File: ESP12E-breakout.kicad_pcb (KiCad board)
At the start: 2 copper layers, 26.7 x 35.1 mm, 17 parts, among them P1 CONN_01X10, P3 CONN_01X08, SW1 RESET, SW2 FLASH, U1 ESP-12E, U2 AP1117

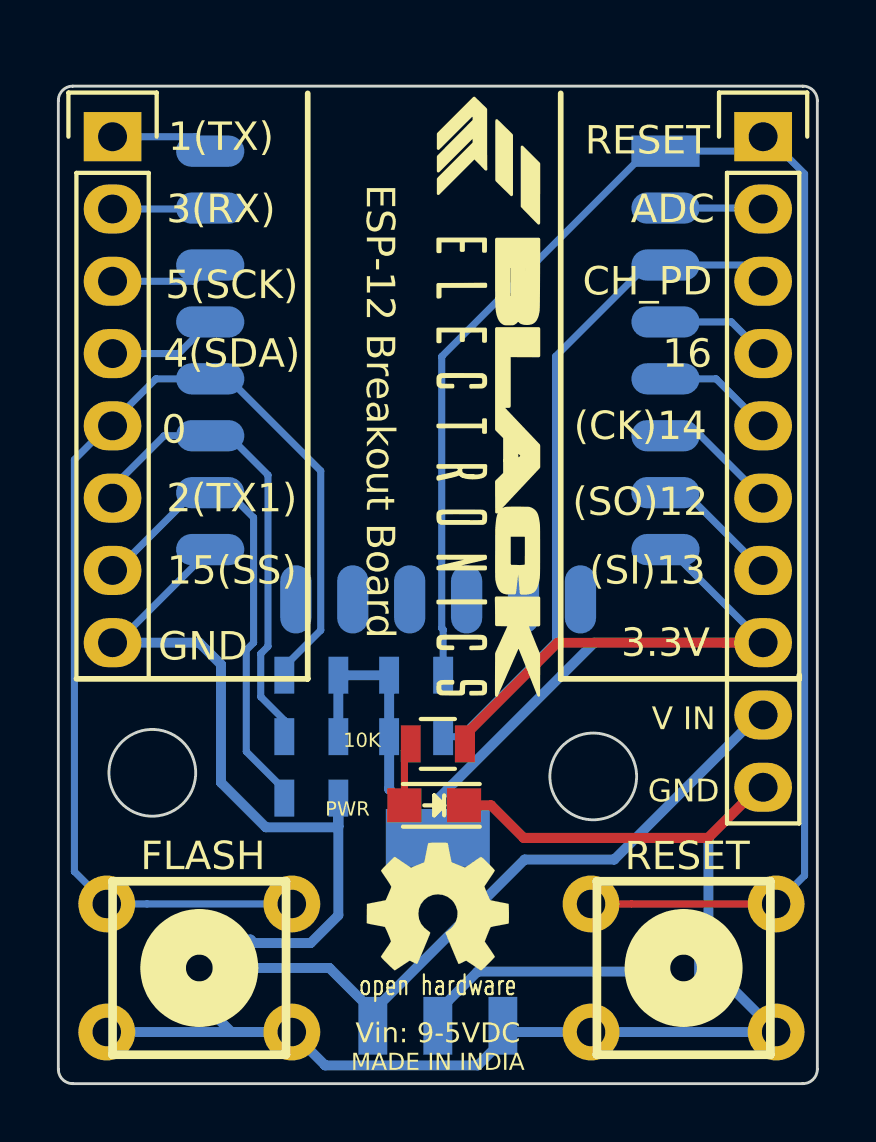
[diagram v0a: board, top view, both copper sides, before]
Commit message: Ready for prototype run
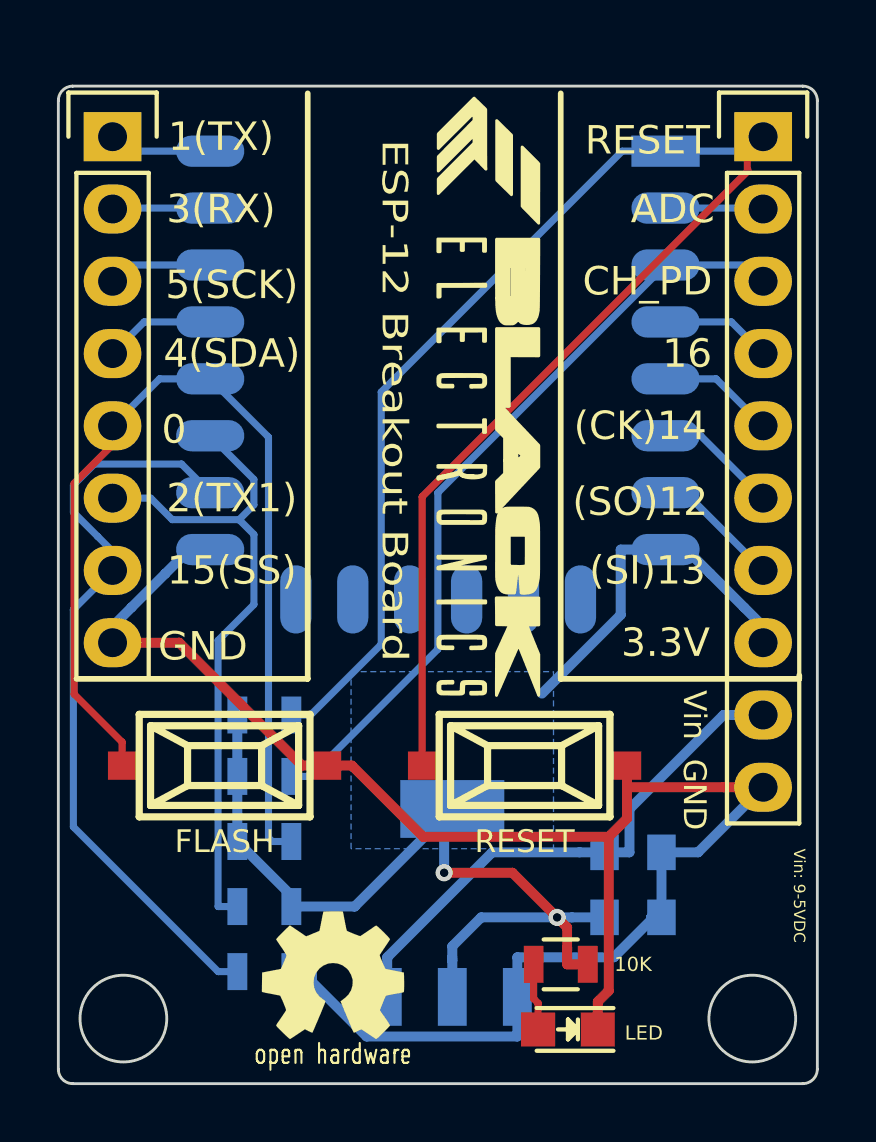
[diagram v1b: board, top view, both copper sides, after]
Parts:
- D1: value PWR -> LED
- SW1, SW2: footprint w_switch:PCB_PUSH_edit -> w_switch:smd_push
- moved C1 15.8 mm to (185.9, 70.9), turned to 0 degrees
- moved D1 9.17 mm to (183.6, 77.1)
- moved SW1 9.04 mm to (182.1, 67.8), turned to 180 degrees
- moved R6 8.87 mm to (183.4, 74.8)
- moved SW2 7.17 mm to (171.6, 67.8), turned to 0 degrees
- moved R5 6.32 mm to (173.0, 75.1)
- moved R4 6.19 mm to (173.0, 72.8)
- moved R3 6.07 mm to (173.0, 70.5), turned to 180 degrees
- moved R1 5.51 mm to (173.0, 66.0)
- moved R2 5.51 mm to (173.0, 68.2)
- moved G1 4.40 mm to (175.4, 75.2)
- moved C2 2.52 mm to (185.9, 73.2)
- moved U2 1.14 mm to (179.6, 72.6)
- renumbered G*** to G0, G*** to G1
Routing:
- net GND: track 82.4 -> 64.4 mm
- net /15: track 17.0 -> 26.5 mm
- net /2: track 16.8 -> 23.6 mm
- net /0: track 41.5 -> 35.1 mm
- net /3V3: track 50.9 -> 44.8 mm, vias 0 -> 2
- net /5V: track 24.3 -> 19.0 mm
- net /CH_PD: track 24.2 -> 27.5 mm
- net /RESET: track 60.3 -> 57.3 mm
- added copper zone on B.Cu, net /3V3
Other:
- outline, holes or cut-outs redrawn
- board text added: "Vin"
- board text removed: "MADE IN INDIA"
- board text removed: "V IN"
